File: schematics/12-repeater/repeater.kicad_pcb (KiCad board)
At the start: 4 copper layers, 53 x 25 mm, 13 parts, among them J1 Cat5, J2 PSG01571, U1 PCA9600D

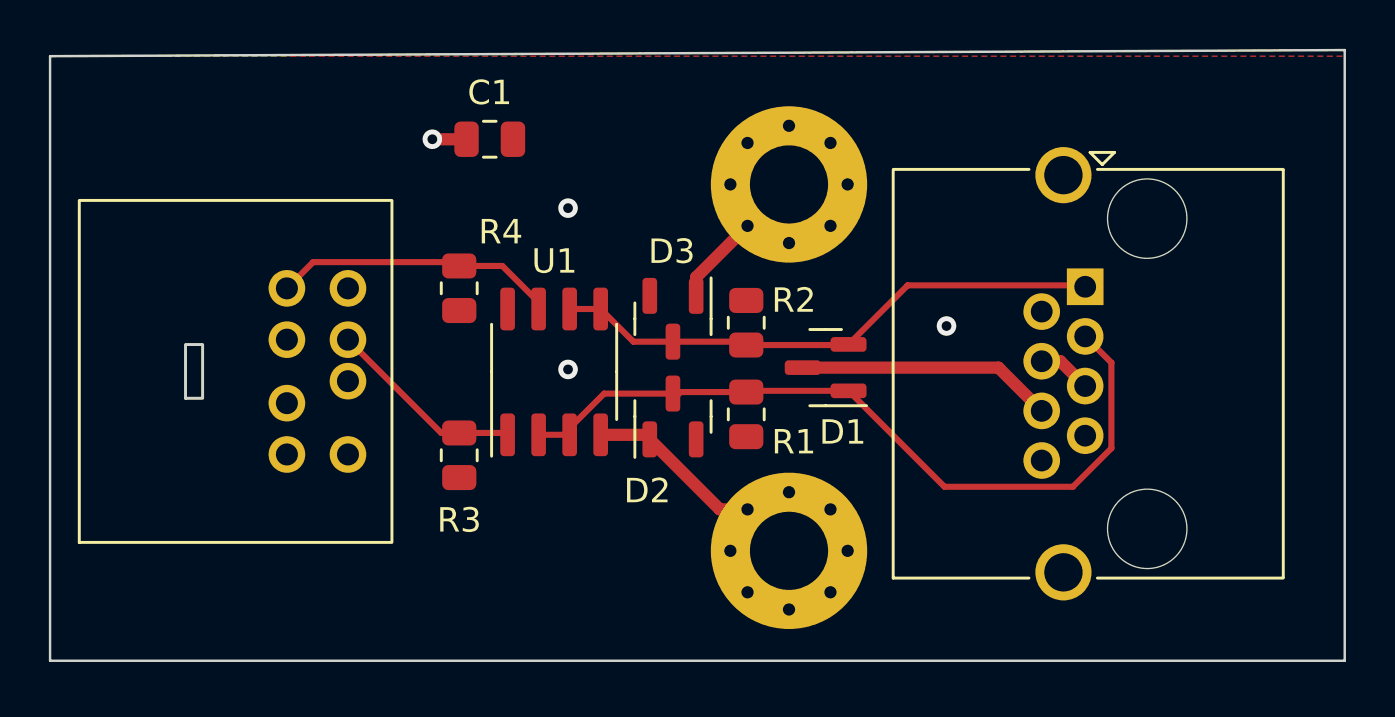
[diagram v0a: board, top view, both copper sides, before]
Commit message: Update repeater ready for manufacture
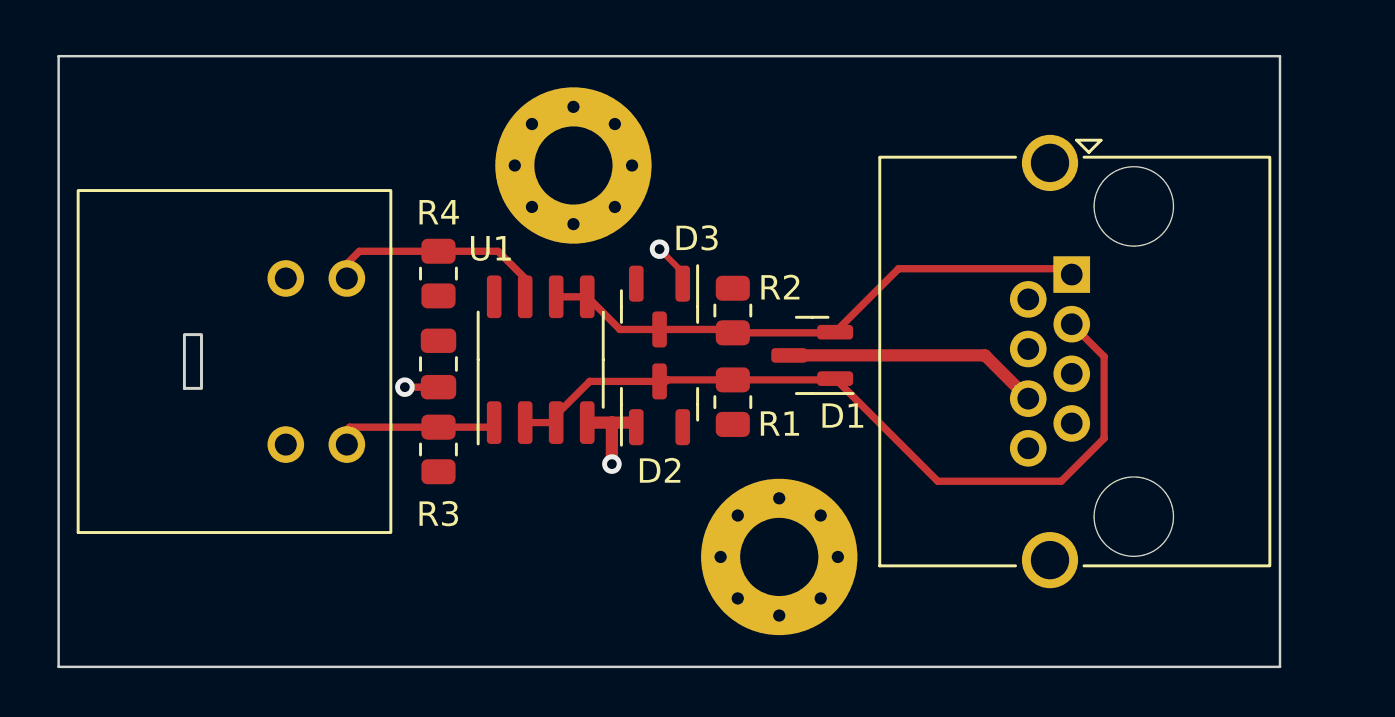
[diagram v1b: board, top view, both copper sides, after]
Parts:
- moved C1 9.44 mm to (134.7, 115.6), turned to -90 degrees
- moved H1 8.86 mm to (140.2, 107.5)
- moved R4 1.04 mm to (134.7, 111.9)
- moved R3 0.88 mm to (134.7, 119.1)
- moved D1 0.74 mm to (149.9, 115.2)
- moved D2 0.74 mm to (143.7, 117.2)
- moved D3 0.74 mm to (143.7, 113.2)
- moved J1 0.74 mm to (160.6, 111.9)
- moved R1 0.74 mm to (146.7, 117.2)
- moved R2 0.74 mm to (146.7, 113.4)
- moved U1 0.74 mm to (138.8, 115.4)
- moved H2 0.47 mm to (148.6, 123.5)
- moved J2 0.41 mm to (119.9, 122.5)
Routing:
- net GND: track 25.3 -> 17.5 mm, vias 1 -> 3
- net /SCL: track 11.7 -> 9.44 mm
- net 1v8: track 2.20 -> 0.00 mm, vias 3 -> 0
- net /SDA: track 8.15 -> 6.87 mm
- net /SDA_D: track 31.8 -> 32.4 mm
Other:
- board size 53 x 25 mm -> 50 x 25 mm
